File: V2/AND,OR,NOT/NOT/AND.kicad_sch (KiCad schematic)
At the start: 15 parts, among them J1 Conn_01x03_Socket, J3 Conn_01x03_Socket, J4 Conn_01x03_Socket, Q1 BSS138, Q2 BSS138, Q3 BSS138, U1 74LVC1G08

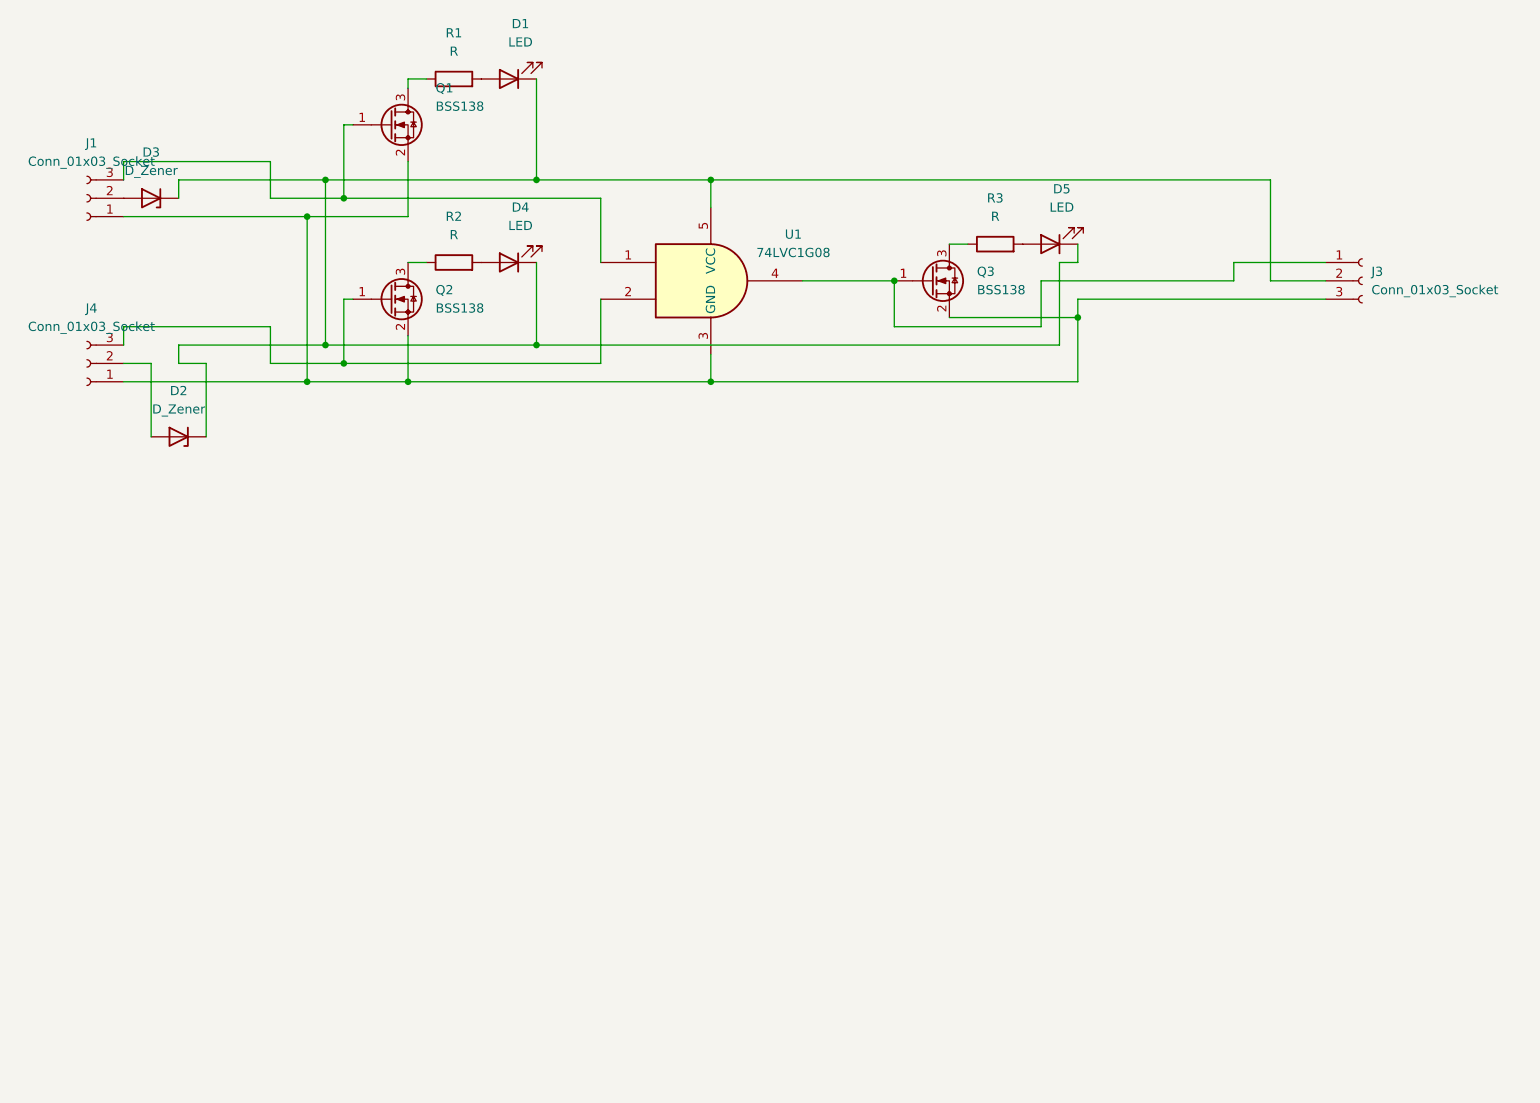
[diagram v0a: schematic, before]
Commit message: fertige Schematik
fertige Schematik
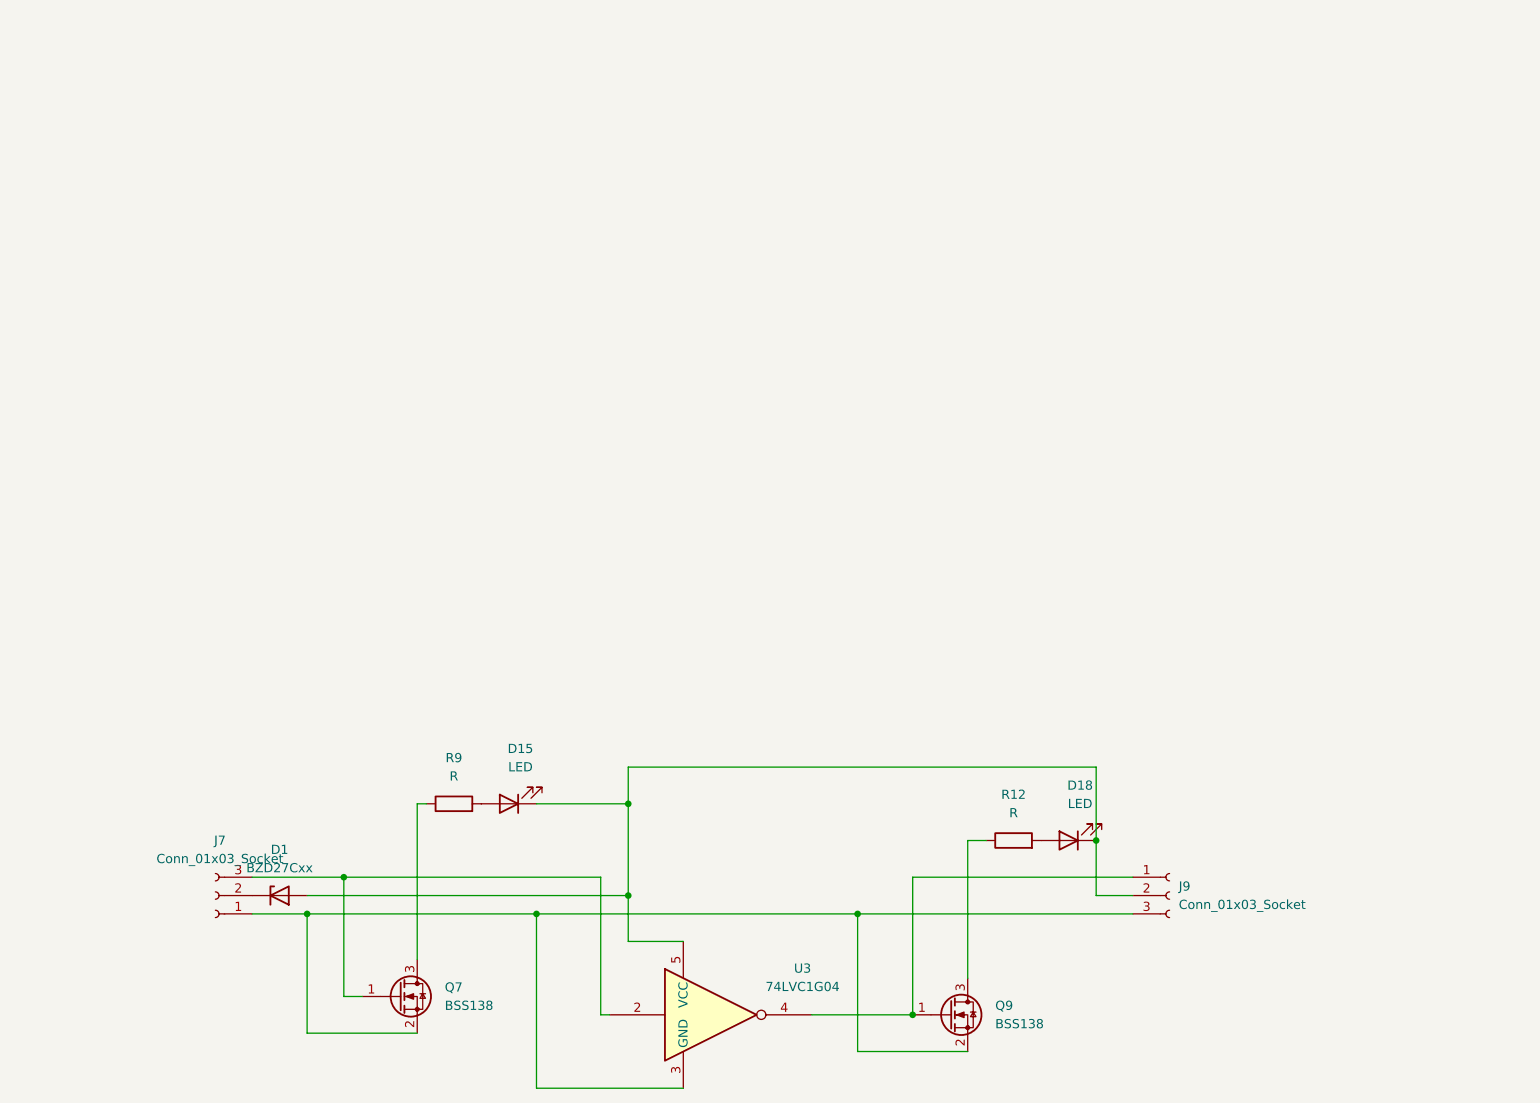
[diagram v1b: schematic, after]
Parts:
- removed D1, D4, D5: LED, LED_SMD:LED_1206_3216Metric, symbol Device:LED
- removed D2, D3: D_Zener, Diode_SMD:D_0201_0603Metric, symbol Device:D_Zener
- removed J1, J3, J4: Conn_01x03_Socket, Connector_PinSocket_2.54mm:PinSocket_1x03_P2.54mm_Horizontal, symbol Connector:Conn_01x03_Socket
- removed Q1, Q2, Q3: BSS138, Package_TO_SOT_SMD:SOT-23, symbol Transistor_FET:BSS138
- removed R1, R2, R3: R, Resistor_SMD:R_0201_0603Metric, symbol Device:R
- removed U1: 74LVC1G08, Package_TO_SOT_SMD:SOT-353_SC-70-5, symbol 74xGxx:74LVC1G08
- added D1: BZD27Cxx, Diode_SMD:D_SMF, symbol Diode:BZD27Cxx
- added D15, D18: LED, LED_SMD:LED_1206_3216Metric, symbol Device:LED
- added J7, J9: Conn_01x03_Socket, Connector_PinSocket_2.54mm:PinSocket_1x03_P2.54mm_Horizontal, symbol Connector:Conn_01x03_Socket
- added Q7, Q9: BSS138, Package_TO_SOT_SMD:SOT-23, symbol Transistor_FET:BSS138
- added R12, R9: R, Resistor_SMD:R_0201_0603Metric, symbol Device:R
- added U3: 74LVC1G04, symbol 74xGxx:74LVC1G04
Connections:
- new net: D1.2 (A), D15.1 (K), D18.1 (K), J9.2 (Pin_2), U3.5 (VCC)
- new net: D15.2 (A), R9.2
- new net: J7.3 (Pin_3), Q7.1 (G), U3.2
- new net: J7.1 (Pin_1), J9.3 (Pin_3), Q7.2 (S), Q9.2 (S), U3.3 (GND)
- new net: Q7.3 (D), R9.1
- new net: Q9.3 (D), R12.1
- new net: D18.2 (A), R12.2
- new net: D1.1 (K), J7.2 (Pin_2)
- new net: J9.1 (Pin_1), Q9.1 (G), U3.4
